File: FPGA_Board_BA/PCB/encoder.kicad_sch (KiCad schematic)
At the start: 7 parts, among them J20 Molex_Mini_Fit_Jr_2x08pin, U16 SN74LXC2T45Q1, U17 SN74LXC2T45Q1

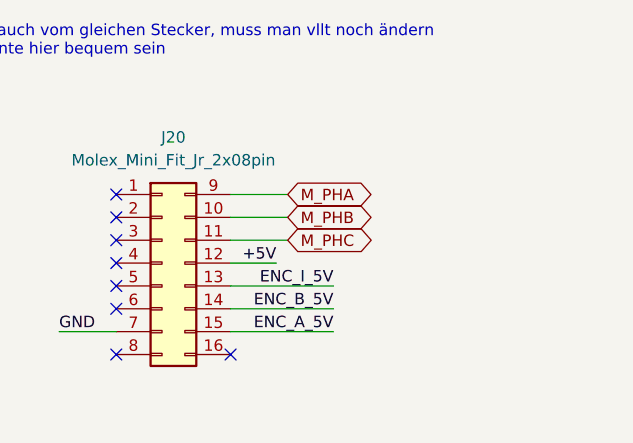
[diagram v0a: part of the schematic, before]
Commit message: Besprechung mit Leo
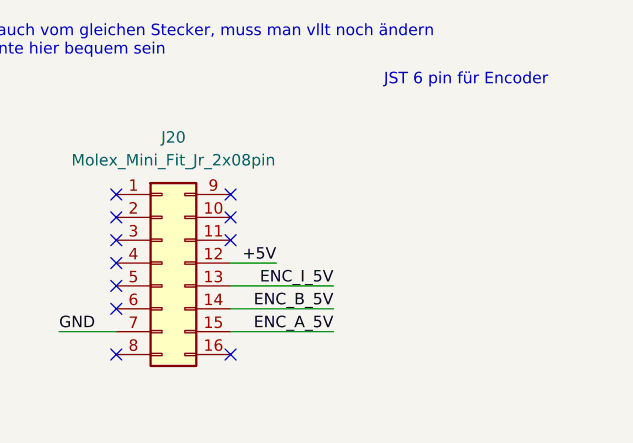
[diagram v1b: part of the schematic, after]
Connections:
- net M_PHA: no longer names the net of J20.9 (Pin_9)
- net M_PHB: no longer names the net of J20.10 (Pin_10)
- net M_PHC: no longer names the net of J20.11 (Pin_11)
- no-connect marks 10 -> 13
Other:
- note added: "JST 6 pin für Encoder"
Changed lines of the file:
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@@
 		)
 	)
+	(text "JST 6 pin für Encoder"
+		(exclude_from_sim no)
+		(at 253.492 24.13 0)
+		(effects
+			(font
+				(size 1.27 1.27)
+			)
+		)
+	)
 	(junction
 		(at 219.71 149.86)
@@
 	)
 	(no_connect
+		(at 227.33 36.83)
+	)
+	(no_connect
 		(at 214.63 46.99)
 	)
@@
 	)
 	(no_connect
+		(at 227.33 41.91)
+	)
+	(no_connect
 		(at 229.87 137.16)
 	)
@@
 	)
 	(no_connect
+		(at 227.33 39.37)
+	)
+	(no_connect
 		(at 214.63 36.83)
 	)
@@
 	(wire
 		(pts
-			(xy 227.33 41.91) (xy 233.68 41.91)
-		)
-		(stroke
-			(width 0)
-			(type default)
-		)
-	)
-	(wire
-		(pts
 			(xy 209.55 142.24) (xy 187.96 142.24)
 		)
@@
 	(wire
 		(pts
-			(xy 227.33 36.83) (xy 233.68 36.83)
-		)
-		(stroke
-			(width 0)
-			(type default)
-		)
-	)
-	(wire
-		(pts
 			(xy 217.17 119.38) (xy 217.17 121.92)
 		)
@@
 	(wire
 		(pts
-			(xy 227.33 39.37) (xy 233.68 39.37)
-		)
-		(stroke
-			(width 0)
-			(type default)
-		)
-	)
-	(wire
-		(pts
 			(xy 238.76 52.07) (xy 227.33 52.07)
 		)
@@
 		)
 	)
-	(global_label "M_PHC"
-		(shape bidirectional)
-		(at 233.68 41.91 0)
-		(fields_autoplaced yes)
-		(effects
-			(font
-				(size 1.27 1.27)
-			)
-			(justify left)
-		)
-		(property "Intersheetrefs" "${INTERSHEET_REFS}"
-			(at 244.066 41.91 0)
-			(effects
-				(font
-					(size 1.27 1.27)
-				)
-				(justify left)
-				(hide yes)
-			)
-		)
-	)
-	(global_label "M_PHB"
-		(shape bidirectional)
-		(at 233.68 39.37 0)
-		(fields_autoplaced yes)
-		(effects
-			(font
-				(size 1.27 1.27)
-			)
-			(justify left)
-		)
-		(property "Intersheetrefs" "${INTERSHEET_REFS}"
-			(at 244.066 39.37 0)
-			(effects
-				(font
-					(size 1.27 1.27)
-				)
-				(justify left)
-				(hide yes)
-			)
-		)
-	)
-	(global_label "M_PHA"
-		(shape bidirectional)
-		(at 233.68 36.83 0)
-		(fields_autoplaced yes)
-		(effects
-			(font
-				(size 1.27 1.27)
-			)
-			(justify left)
-		)
-		(property "Intersheetrefs" "${INTERSHEET_REFS}"
-			(at 243.8846 36.83 0)
-			(effects
-				(font
-					(size 1.27 1.27)
-				)
-				(justify left)
-				(hide yes)
-			)
-		)
-	)

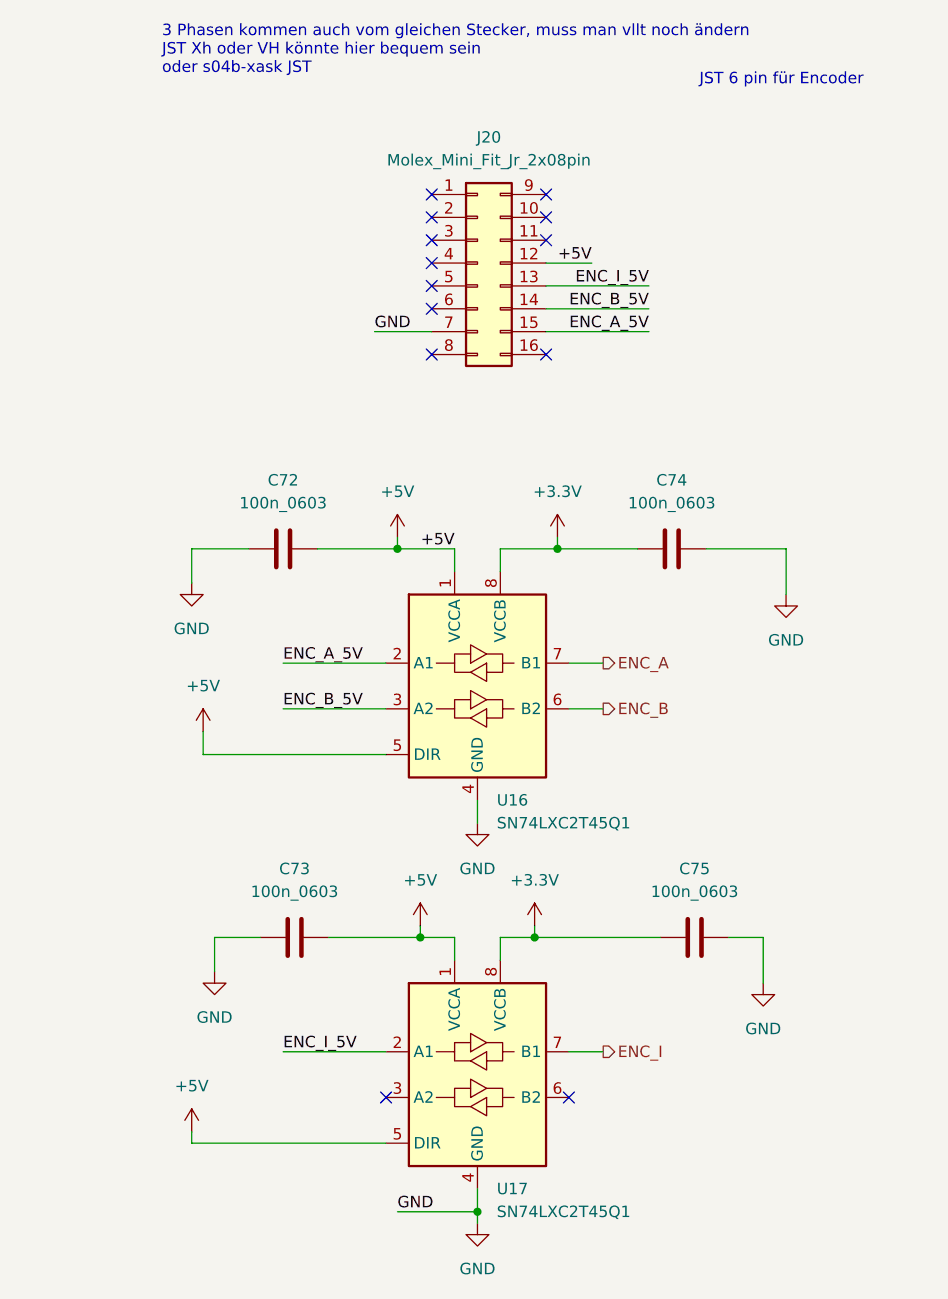
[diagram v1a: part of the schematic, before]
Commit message: 22.11
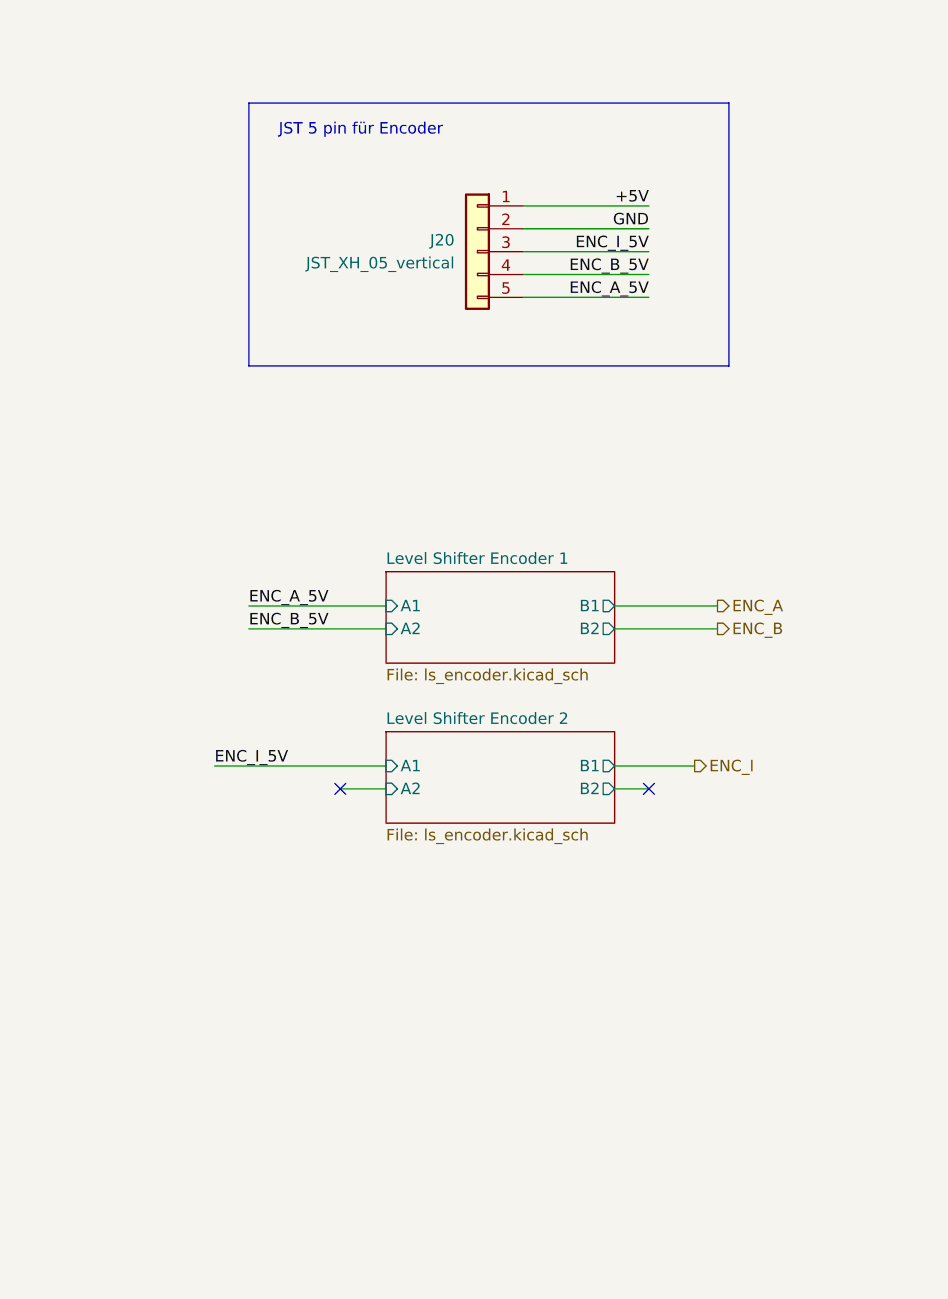
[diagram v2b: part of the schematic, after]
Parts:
- removed C72, C73, C74, C75: 100n_0603, WLIB_Capacitor:C_0603, symbol WLIB_C:100n_0603
- removed J20: Molex_Mini_Fit_Jr_2x08pin, MYLIB_Misc:Molex_2x8pin_vertical_tht, symbol MYLIB_Misc:Molex_Mini_Fit_Jr_2x08
- removed U16, U17: SN74LXC2T45Q1, MYLIB_Misc:SN74LXC2T45QDCURQ1, symbol MYLIB_Misc:SN74LXC2T45Q1
- added J20: JST_XH_05_vertical, Connector_JST:JST_XH_B5B-XH-A_1x05_P2.50mm_Vertical, symbol WLIB_J:JST_XH_05_vertical
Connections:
- net +5V: now also J20.1 (Pin_1)
- net ENC_A_5V: now also J20.5 (Pin_5)
- net ENC_B_5V: now also J20.4 (Pin_4)
- net ENC_I_5V: now also J20.3 (Pin_3)
- net GND: now also J20.2 (Pin_2)
- no-connect marks 13 -> 2
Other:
- added sheet Level Shifter Encoder 1 (ls_encoder.kicad_sch)
- added sheet Level Shifter Encoder 2 (ls_encoder.kicad_sch)
- note added: "JST 5 pin für Encoder"
- note removed: "3 Phasen kommen auch vom gleichen Stecker, muss man vllt noch ändern JST Xh oder VH könnte hier bequem sein oder s04b-xask JST"
- note removed: "JST 6 pin für Encoder"
